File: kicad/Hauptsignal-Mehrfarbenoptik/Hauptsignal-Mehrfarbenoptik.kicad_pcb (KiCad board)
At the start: 2 copper layers, 6.6 x 13.6 mm, 17 parts, among them J0 VCC, J1 VkzBw, J2 ARGB_2, J3 ARGB_3, J4 ARGB_4, J5 Zs7-3, J6 Ra, J7 Zs7-1, J8 Zs7-2, J9 Ra/Zs1

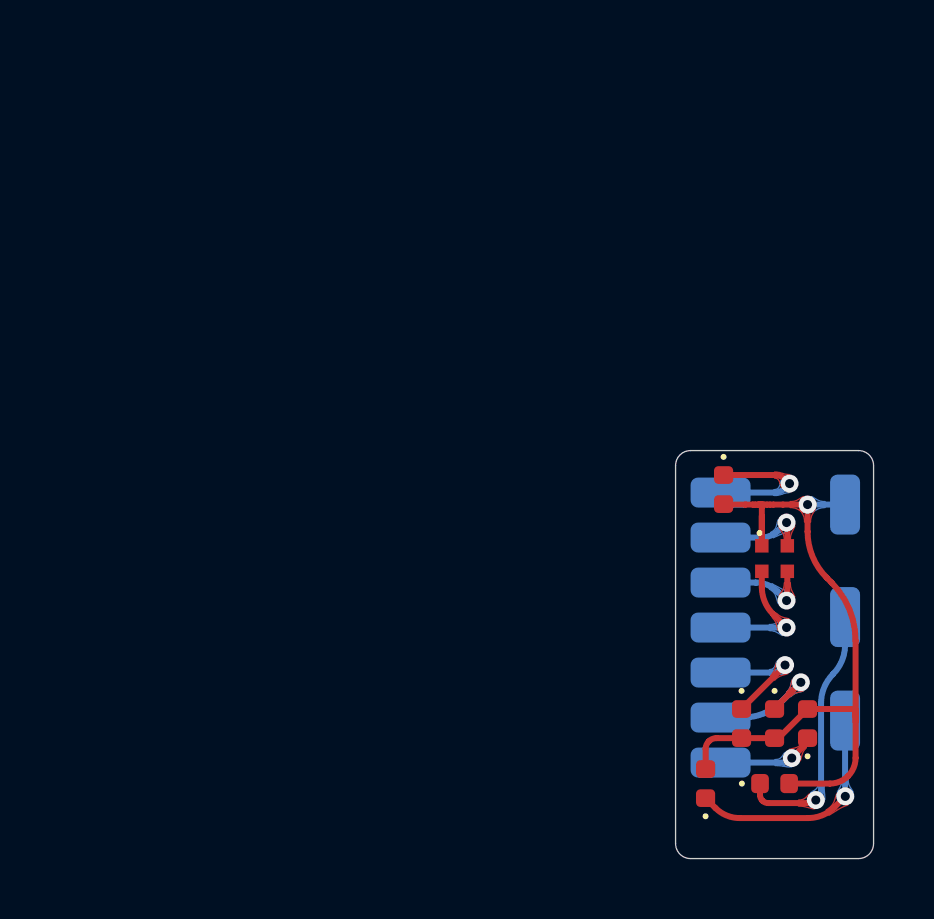
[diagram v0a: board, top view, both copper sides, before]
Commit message: Add CC-BY-SA 4.0 license
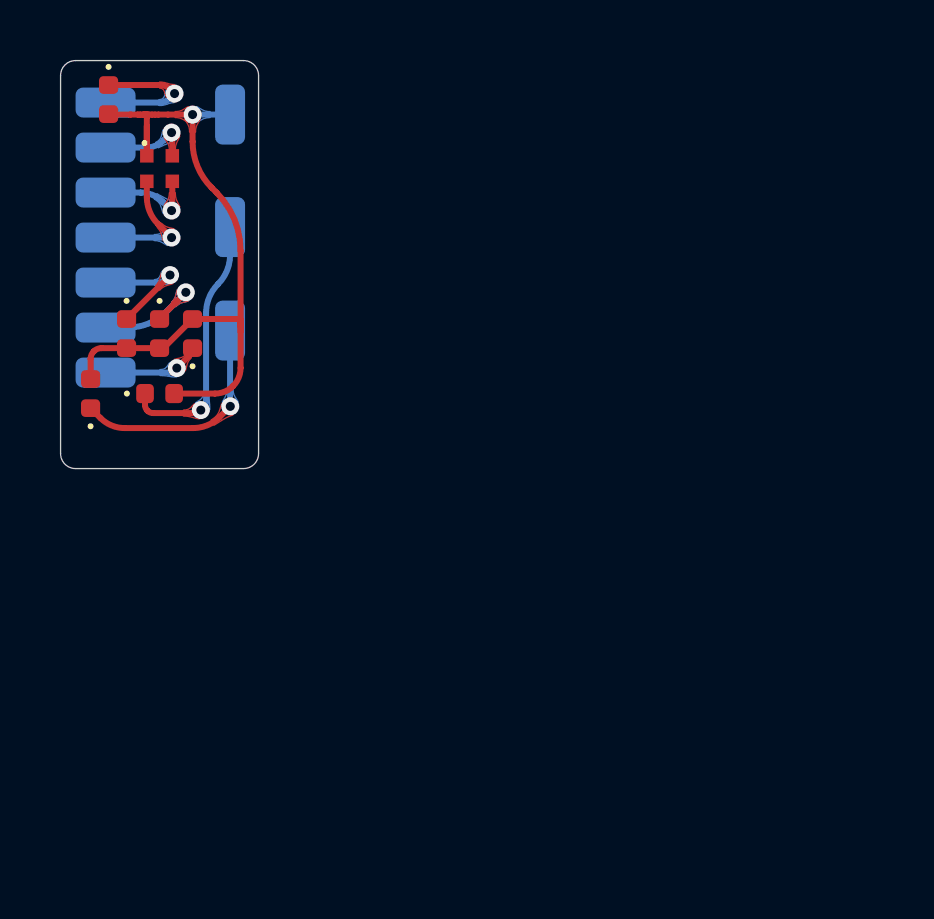
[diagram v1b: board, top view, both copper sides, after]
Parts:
- moved J1 24.3 mm to (101.0, 61.4)
- moved J2 24.3 mm to (101.0, 62.9)
- moved D1 24.3 mm to (101.1, 61.3)
- moved D10 24.3 mm to (100.5, 71.1)
- moved D6 24.3 mm to (101.7, 69.1)
- moved D7 24.3 mm to (102.8, 69.1)
- moved D8 24.3 mm to (103.9, 69.1)
- moved D9 24.3 mm to (102.8, 71.1)
- moved J0 24.3 mm to (105.2, 61.8)
- moved J3 24.3 mm to (101.0, 64.4)
- moved J4 24.3 mm to (101.0, 65.9)
- moved J5 24.3 mm to (101.0, 67.4)
- moved J6 24.3 mm to (101.0, 68.9)
- moved J7 24.3 mm to (101.0, 70.4)
- moved J8 24.3 mm to (105.2, 65.5)
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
